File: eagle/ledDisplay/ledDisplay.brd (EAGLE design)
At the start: 68.6 x 92.7 mm, 80 parts, among them IC4 MCP1703CB, U1 PCA9685

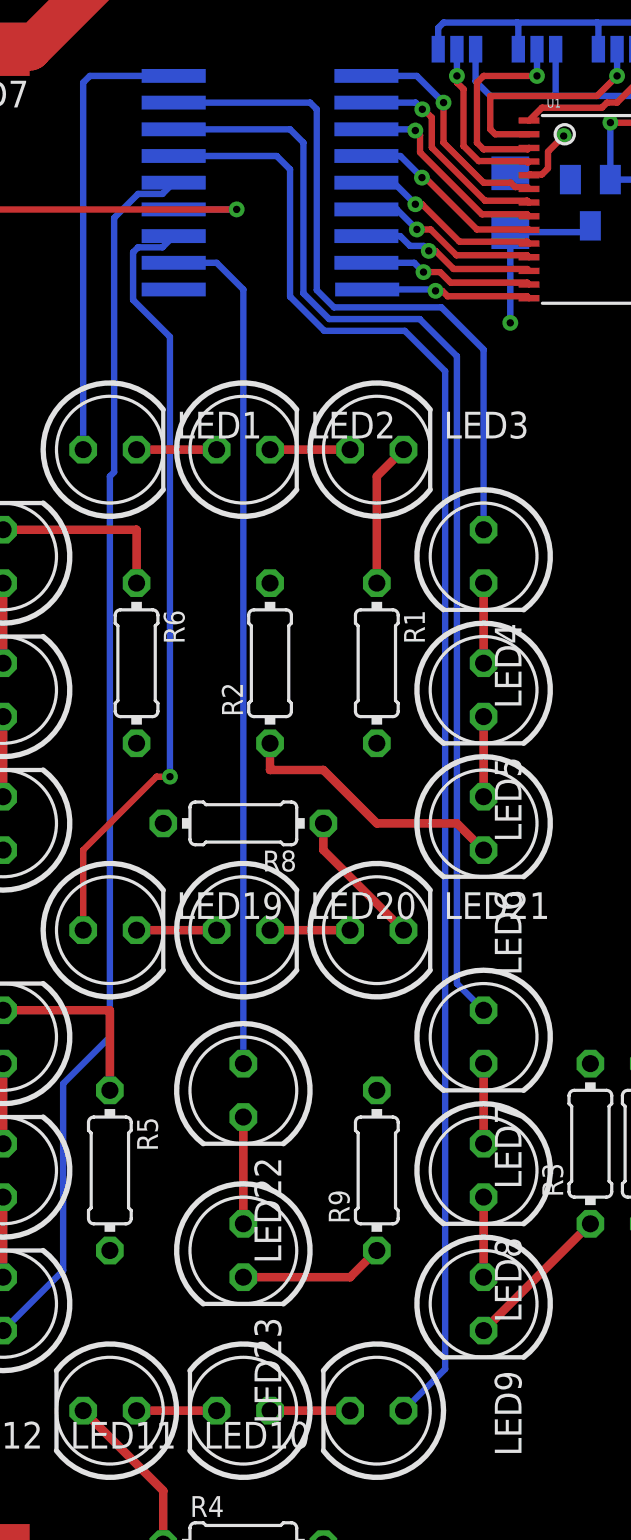
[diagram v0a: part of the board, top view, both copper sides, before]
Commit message: hole git (feat): synced github with school server
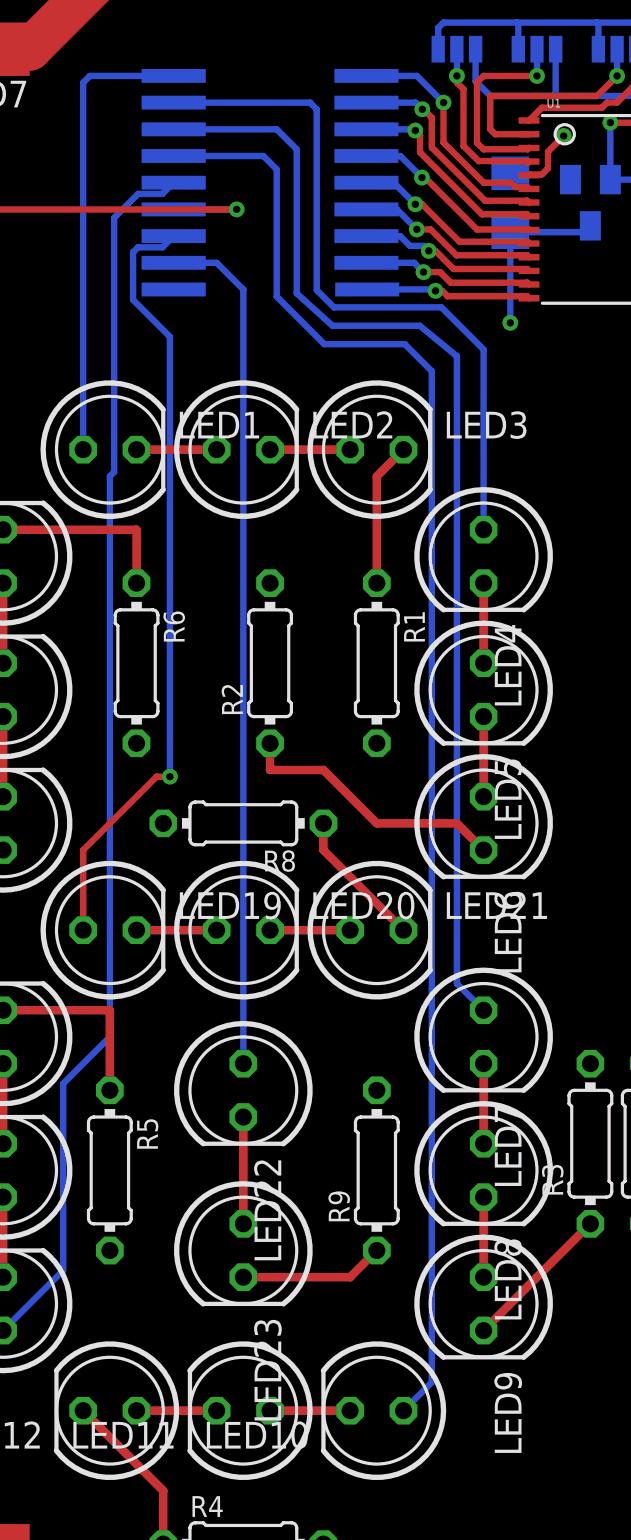
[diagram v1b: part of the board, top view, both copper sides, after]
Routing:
- net N$19: track 71.0 -> 70.1 mm
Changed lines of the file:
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@@
 <?xml version="1.0" encoding="utf-8"?>
 <!DOCTYPE eagle SYSTEM "eagle.dtd">
-<eagle version="8.3.2">
+<eagle version="8.4.0">
 <drawing>
 <settings>
@@
 <param name="dpMaxLengthDifference" value="10mm"/>
 <param name="dpGapFactor" value="2.5"/>
-<param name="checkGrid" value="0"/>
-<param name="checkAngle" value="0"/>
 <param name="checkFont" value="1"/>
 <param name="checkRestrict" value="1"/>
+<param name="checkStop" value="0"/>
 <param name="useDiameter" value="13"/>
 <param name="maxErrors" value="50"/>
@@
 <contactref element="IC1" pad="16"/>
 <contactref element="LED7" pad="A"/>
-<wire x1="13.1954" y1="78.74" x2="18.7325" y2="78.74" width="0.3048" layer="16"/>
-<wire x1="18.7325" y1="78.74" x2="19.3675" y2="78.105" width="0.3048" layer="16"/>
-<wire x1="24.903025" y1="69.711975" x2="26.67" y2="67.945" width="0.3048" layer="16"/>
-<wire x1="20.59161875" y1="69.711975" x2="24.903025" y2="69.711975" width="0.3048" layer="16"/>
-<wire x1="19.3675" y1="78.105" x2="19.3675" y2="70.93609375" width="0.3048" layer="16"/>
-<wire x1="19.3675" y1="70.93609375" x2="20.59161875" y2="69.711975" width="0.3048" layer="16"/>
+<wire x1="13.1954" y1="78.74" x2="18.0975" y2="78.74" width="0.3048" layer="16"/>
+<wire x1="18.0975" y1="78.74" x2="19.05" y2="77.7875" width="0.3048" layer="16"/>
+<wire x1="24.903025" y1="69.394475" x2="26.67" y2="67.945" width="0.3048" layer="16"/>
+<wire x1="20.75036875" y1="69.394475" x2="24.903025" y2="69.394475" width="0.3048" layer="16"/>
+<wire x1="19.05" y1="77.7875" x2="19.05" y2="70.93609375" width="0.3048" layer="16"/>
+<wire x1="19.05" y1="70.93609375" x2="20.75036875" y2="69.394475" width="0.3048" layer="16"/>
 <wire x1="26.67" y1="67.945" x2="26.67" y2="38.1" width="0.3048" layer="16"/>
 <wire x1="26.67" y1="38.1" x2="27.94" y2="36.83" width="0.3048" layer="16"/>
@@
 <contactref element="IC1" pad="15"/>
 <contactref element="LED10" pad="A"/>
-<wire x1="13.1953" y1="77.47" x2="18.0975" y2="77.47" width="0.3048" layer="16"/>
-<wire x1="18.0975" y1="77.47" x2="18.7325" y2="76.835" width="0.3048" layer="16"/>
-<wire x1="24.191825" y1="69.153175" x2="26.1112" y2="67.2338" width="0.3048" layer="16"/>
-<wire x1="20.36015" y1="69.153175" x2="24.191825" y2="69.153175" width="0.3048" layer="16"/>
-<wire x1="18.7325" y1="76.835" x2="18.7325" y2="70.780825" width="0.3048" layer="16"/>
-<wire x1="18.7325" y1="70.780825" x2="20.36015" y2="69.153175" width="0.3048" layer="16"/>
-<wire x1="26.1112" y1="67.2338" x2="26.1112" y2="19.7612" width="0.3048" layer="16"/>
-<wire x1="26.1112" y1="19.7612" x2="24.13" y2="17.78" width="0.3048" layer="16"/>
+<wire x1="13.1953" y1="77.47" x2="17.4625" y2="77.47" width="0.3048" layer="16"/>
+<wire x1="17.4625" y1="77.47" x2="18.0975" y2="76.835" width="0.3048" layer="16"/>
+<wire x1="24.191825" y1="68.518175" x2="25.4762" y2="67.2338" width="0.3048" layer="16"/>
+<wire x1="20.36015" y1="68.518175" x2="24.191825" y2="68.518175" width="0.3048" layer="16"/>
+<wire x1="18.0975" y1="76.835" x2="18.0975" y2="70.780825" width="0.3048" layer="16"/>
+<wire x1="18.0975" y1="70.780825" x2="20.36015" y2="68.518175" width="0.3048" layer="16"/>
+<wire x1="25.4762" y1="67.2338" x2="25.4762" y2="19.1262" width="0.3048" layer="16"/>
+<wire x1="25.4762" y1="19.1262" x2="24.13" y2="17.78" width="0.3048" layer="16"/>
 </signal>
 <signal name="+12V">
